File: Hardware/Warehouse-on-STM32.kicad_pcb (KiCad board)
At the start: 2 copper layers, 57 x 47 mm, 79 parts, among them J1 ESP8266, J2 Conn_01x05, J3 Barrel_Jack_Switch, J4 Conn_01x02, J5 Conn_01x02, J6 Conn_01x02, Q1 AO3400A, Q2 AO3400A, SW1 SW_Push, SW2 SW_Push, SW3 SW_Push, SW4 SW_Push, U1 STM32F103C8Tx, U2 EA3036C, U3 MP2225GJ, U4 DRV8820DSG, U5 DRV8820DSG, U6 DRV8820DSG, U7 AHT20, U8 SGP30, U9 Sensor, Y1 Crystal

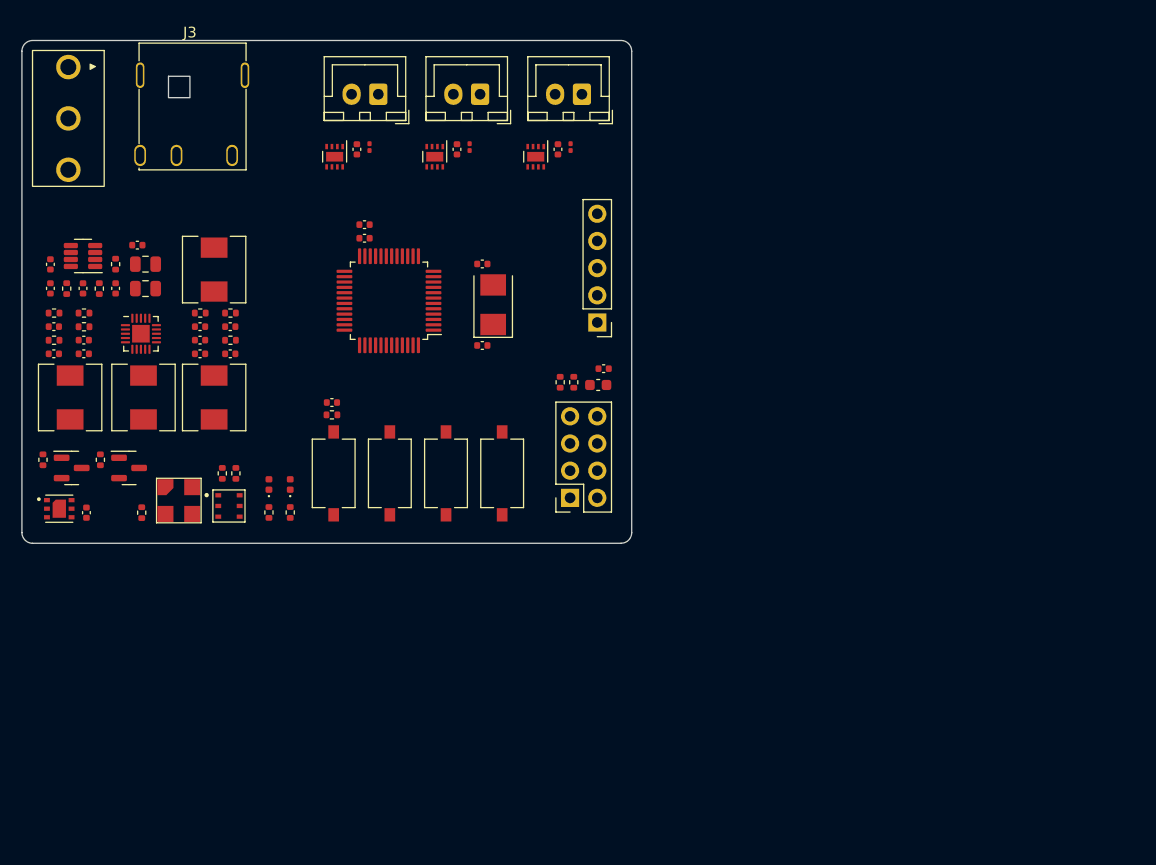
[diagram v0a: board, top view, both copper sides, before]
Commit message: 完成布局
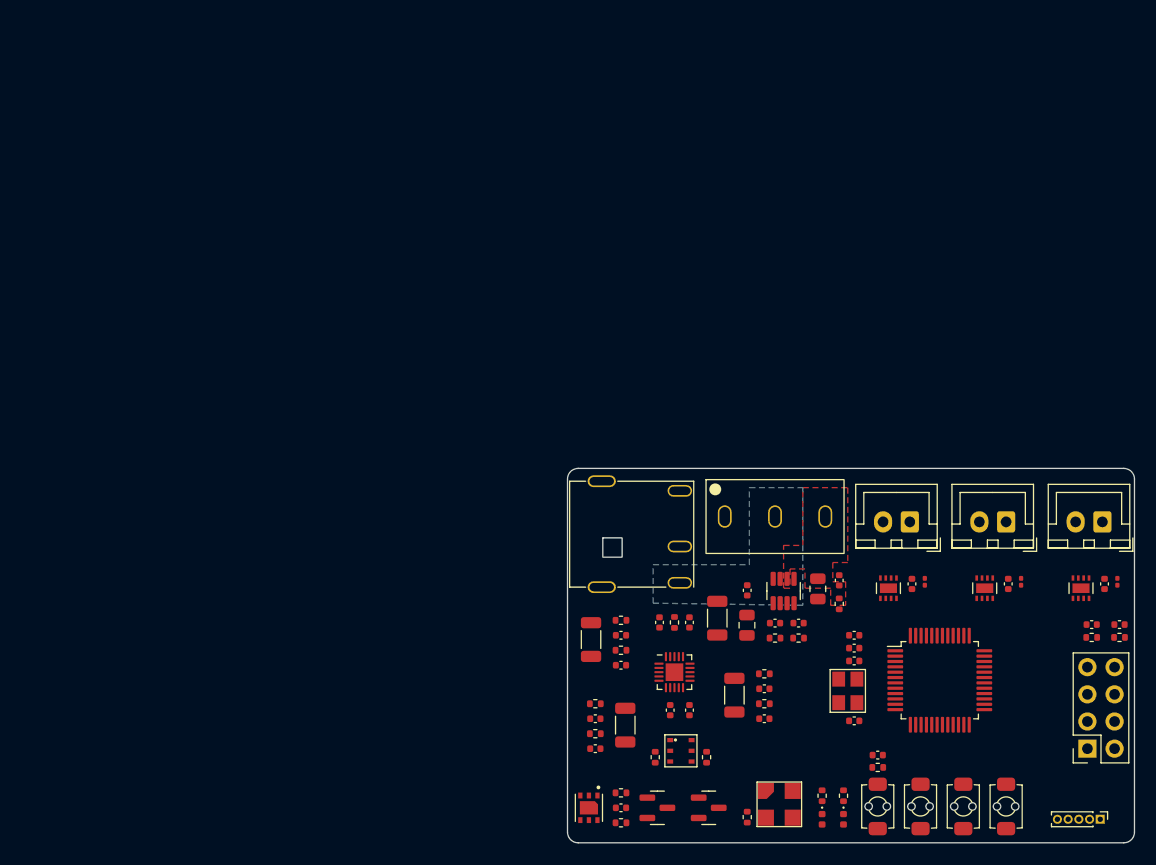
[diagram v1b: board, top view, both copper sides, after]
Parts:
- C1: footprint Capacitor_SMD:C_0603_1608Metric -> Capacitor_SMD:C_0402_1005Metric
- J2: footprint Connector_PinHeader_2.54mm:PinHeader_1x05_P2.54mm_Vertical -> Connector_PinHeader_1.00mm:PinHeader_1x05_P1.00mm_Vertical
- J3: value Barrel_Jack_Switch -> Barrel_Jack_Switch_MountingPin
- L1, L2, L3, L4: footprint Inductor_SMD:L_Chilisin_BMRA00050520 -> Inductor_SMD:L_1206_3216Metric
- SW1, SW2, SW3, SW4: footprint Button_Switch_SMD:SW_Tactile_SPST_NO_Straight_CK_PTS636Sx25SMTRLFS -> Button_Switch_SMD:SW_XKB_TS-1185-B-A-B-A
- SW5: footprint Library:SW -> Button_Switch_THT:SW_XKB_SS-12D10L5
- U7: footprint My_Sensor:AHT20 -> Sensor:AHT20
- U8: footprint My_Sensor:SGP30 -> Sensor:SGP30
- U9: footprint My_Sensor:MEMS气体传感器 -> Sensor:MEMS气体传感器
- Y1: value Crystal -> 8MHz; footprint Crystal:Crystal_SMD_5032-2Pin_5.0x3.2mm -> Crystal:Crystal_SMD_3225-4Pin_3.2x2.5mm
- moved SW5 75.8 mm to (119.4, 104.5), turned to 0 degrees
- moved R13 74.7 mm to (125.4, 112.7), turned to -90 degrees
- moved C20 74.6 mm to (119.4, 114.5), turned to 0 degrees
- moved C22 73.8 mm to (121.6, 114.5), turned to 180 degrees
- moved R15 73.8 mm to (119.4, 115.9), turned to 180 degrees
- moved R14 73.1 mm to (121.6, 115.9), turned to 180 degrees
- moved C19 72.7 mm to (125.4, 110.5), turned to 90 degrees
- moved U3 72.6 mm to (120.2, 111.5), turned to -90 degrees
- moved C21 71.9 mm to (116.8, 111.4)
- moved C17 69.8 mm to (123.4, 111.3), turned to -90 degrees
- moved Q2 67.5 mm to (113.2, 131.7)
- moved J2 66.1 mm to (149.8, 132.8), turned to -90 degrees
- moved C24 65.9 mm to (133.4, 110.6)
- moved C27 65.9 mm to (132.2, 110.8)
- moved C25 65.6 mm to (142.4, 110.6)
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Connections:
- C13 pad 2: Net-(U2-LX3) -> Net-(U2-FB3)
- J2 pad 1: /SWDIO -> /SWCLK
- J2 pad 2: /SWCLK -> /SWDIO
- J2 pad 4: /USART1_TX -> /USART1_RX
- J2 pad 5: /USART1_RX -> /USART1_TX
- L3 pad 2: Net-(U2-FB3) -> Net-(U2-LX3)
- R10 pad 2: Net-(U2-LX3) -> Net-(U2-FB3)
- R11 pad 2: Net-(U2-LX3) -> Net-(U2-FB3)
- U1 pad 14: unconnected-(U1-PA4-Pad14) -> /KEY2
- U1 pad 15: unconnected-(U1-PA5-Pad15) -> /KEY1
- U1 pad 16: /ASLEEP -> /KEY0
- U1 pad 17: /APH -> unconnected-(U1-PA7-Pad17)
- U1 pad 2: /KEY0 -> /ASLEEP
- U1 pad 21: /USART1_RX -> unconnected-(U1-PB10-Pad21)
- U1 pad 29: /AEN -> unconnected-(U1-PA8-Pad29)
- U1 pad 3: /KEY1 -> /APH
- U1 pad 30: /BSLEEP -> /USART1_TX
- U1 pad 31: /BEN -> /USART1_RX
- U1 pad 32: /CSLEEP -> unconnected-(U1-PA11-Pad32)
- U1 pad 33: /CEN -> unconnected-(U1-PA12-Pad33)
- U1 pad 38: unconnected-(U1-PA15-Pad38) -> /CSLEEP
- U1 pad 39: unconnected-(U1-PB3-Pad39) -> /CEN
- U1 pad 4: /KEY2 -> /AEN
- U1 pad 40: unconnected-(U1-PB4-Pad40) -> /BSLEEP
- U1 pad 41: unconnected-(U1-PB5-Pad41) -> /BEN
- U1 pad 46: /USART1_TX -> unconnected-(U1-PB9-Pad46)
- Y1 pad 2: Net-(U1-PD1) -> GND
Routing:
- added copper zone on F.Cu, net +12V
- added copper zone on B.Cu, net Net-(J3-Pad1)
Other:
- board size 57 x 47 mm -> 53 x 35 mm
